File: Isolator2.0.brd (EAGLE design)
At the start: 79.5 x 42.1 mm, 30 parts, among them IC1 MEGA8-AI, IC2 RS485SOIC, J1 RJ45-8PTH, J2 RJ45-8PTH, T3 BC847ALT1SMD

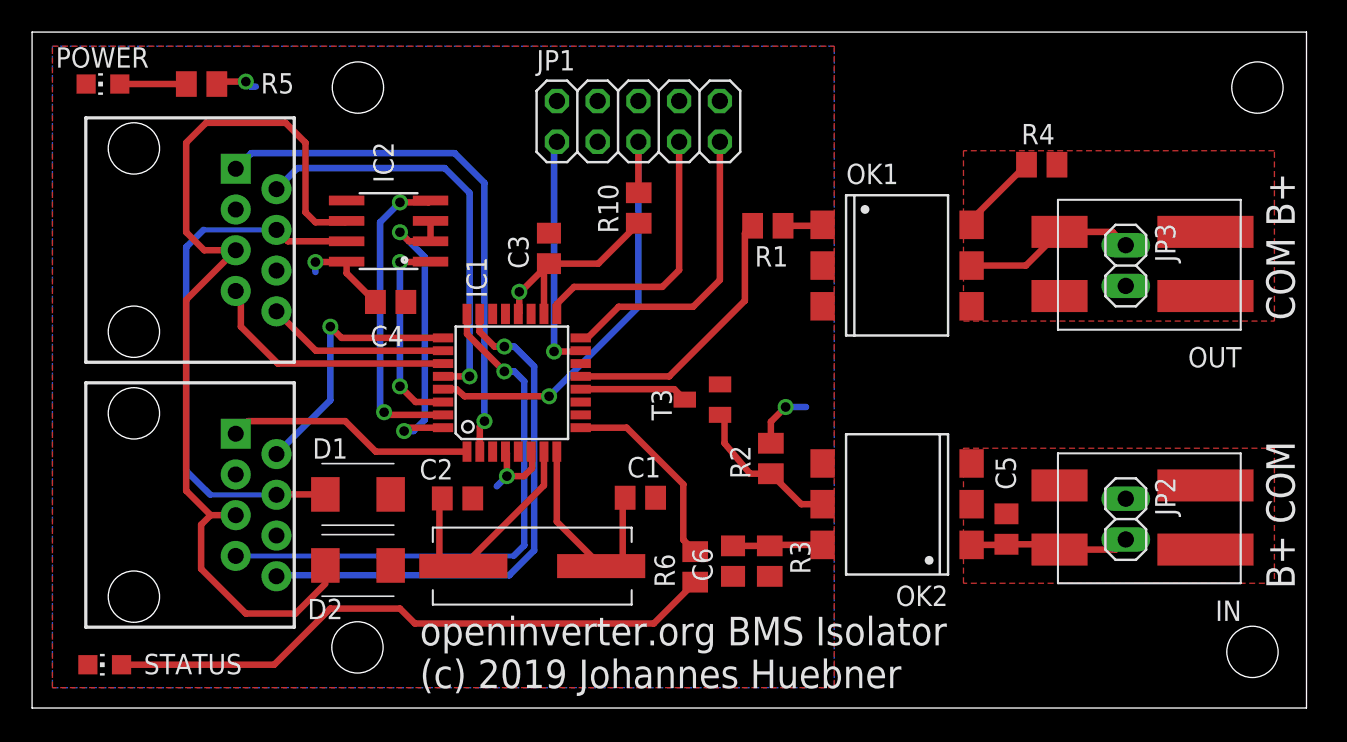
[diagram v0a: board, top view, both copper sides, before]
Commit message: Updated Isolator board and added manufacturing files
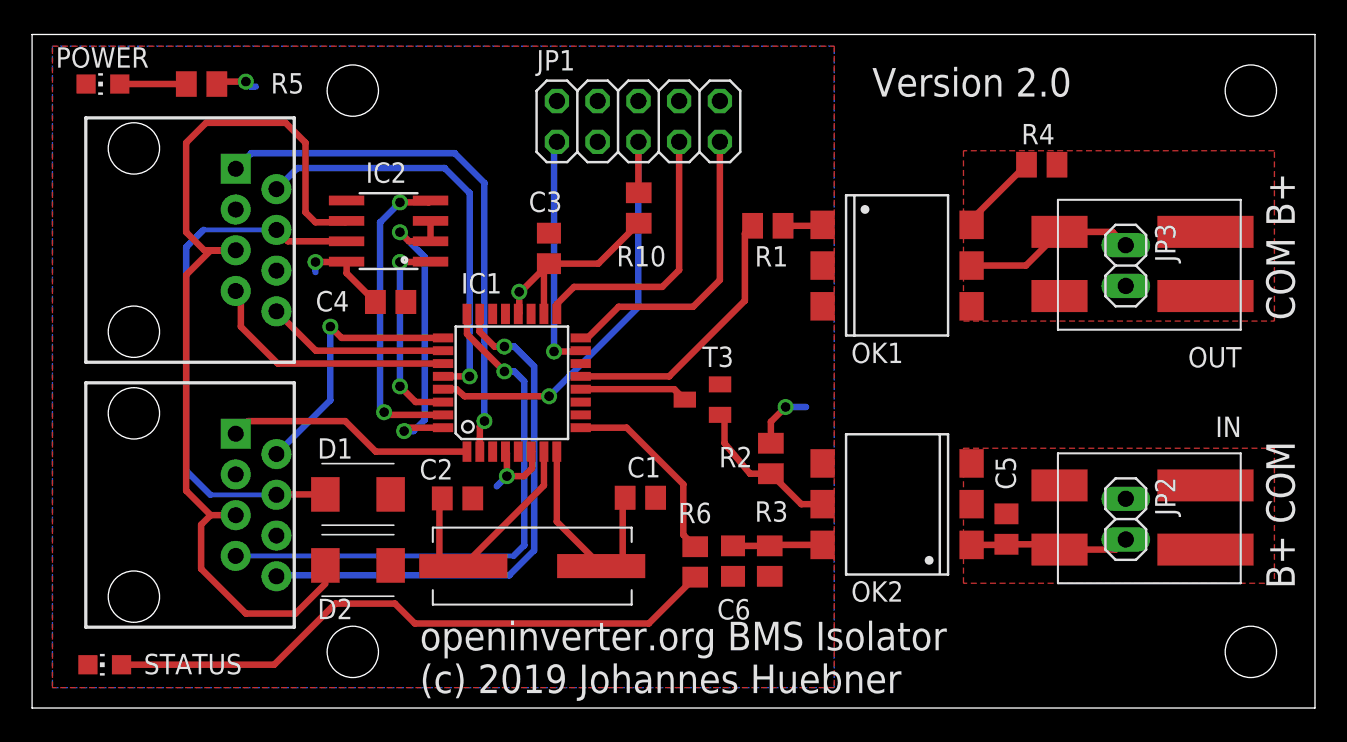
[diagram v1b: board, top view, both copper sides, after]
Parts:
- moved R6 0.31 mm to (41.4, 9.11)
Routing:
- net N$7: track 59.2 -> 60.1 mm
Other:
- board size 79.5 x 42.1 mm -> 80 x 42 mm
- board text added: "Version 2.0"
